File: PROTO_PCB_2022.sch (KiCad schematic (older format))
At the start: 19 parts, among them J1 HORN_EN1, J10 VESC_EN_SIGNAL, J11 BRAKELIGHTS_PWR_OUT, J12 HORN_PWR_OUT, J2 BRAKELIGHTS_EN1, J3 STARTER_MOTOR_EN, J4 12V_BATT1, J5 12V_EXTRA, J6 ECU_POWER_DIST, J7 ECU_KILL_1, J8 ECU_KILL_2, J9 ECU_KILL_3, K1 RT214012, Q1 BRAKELIGHTS_MOSFET1, Q2 HORN_MOSFET1

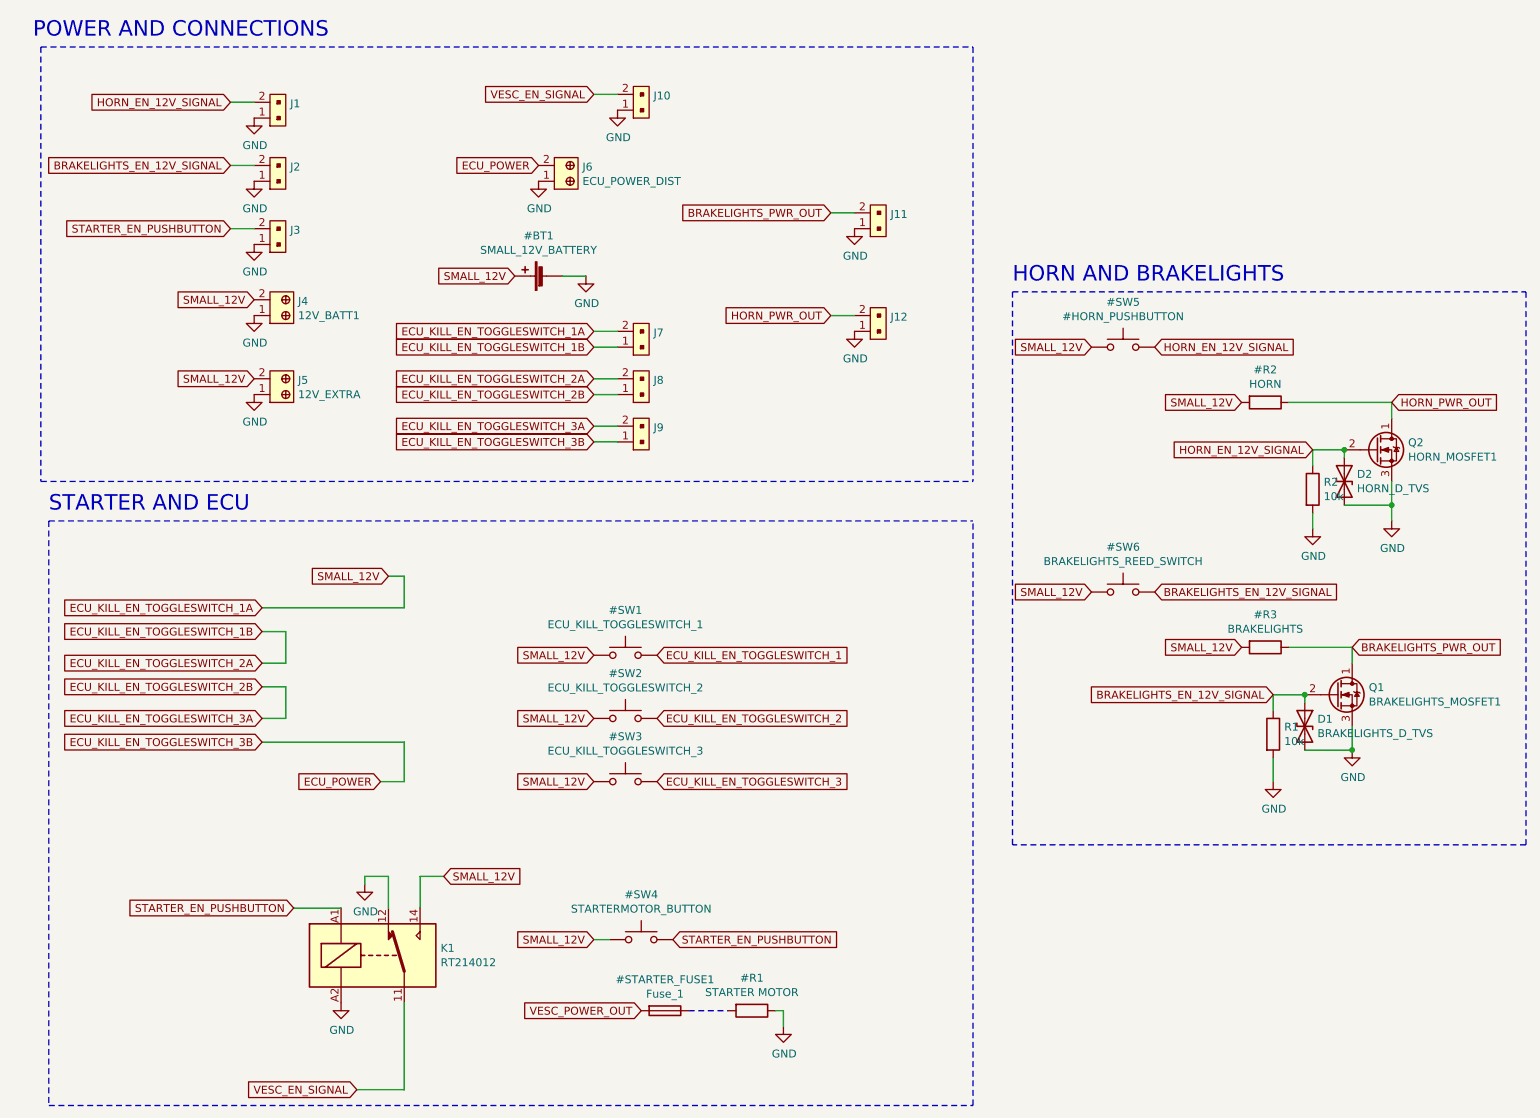
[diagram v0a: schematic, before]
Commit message: second version
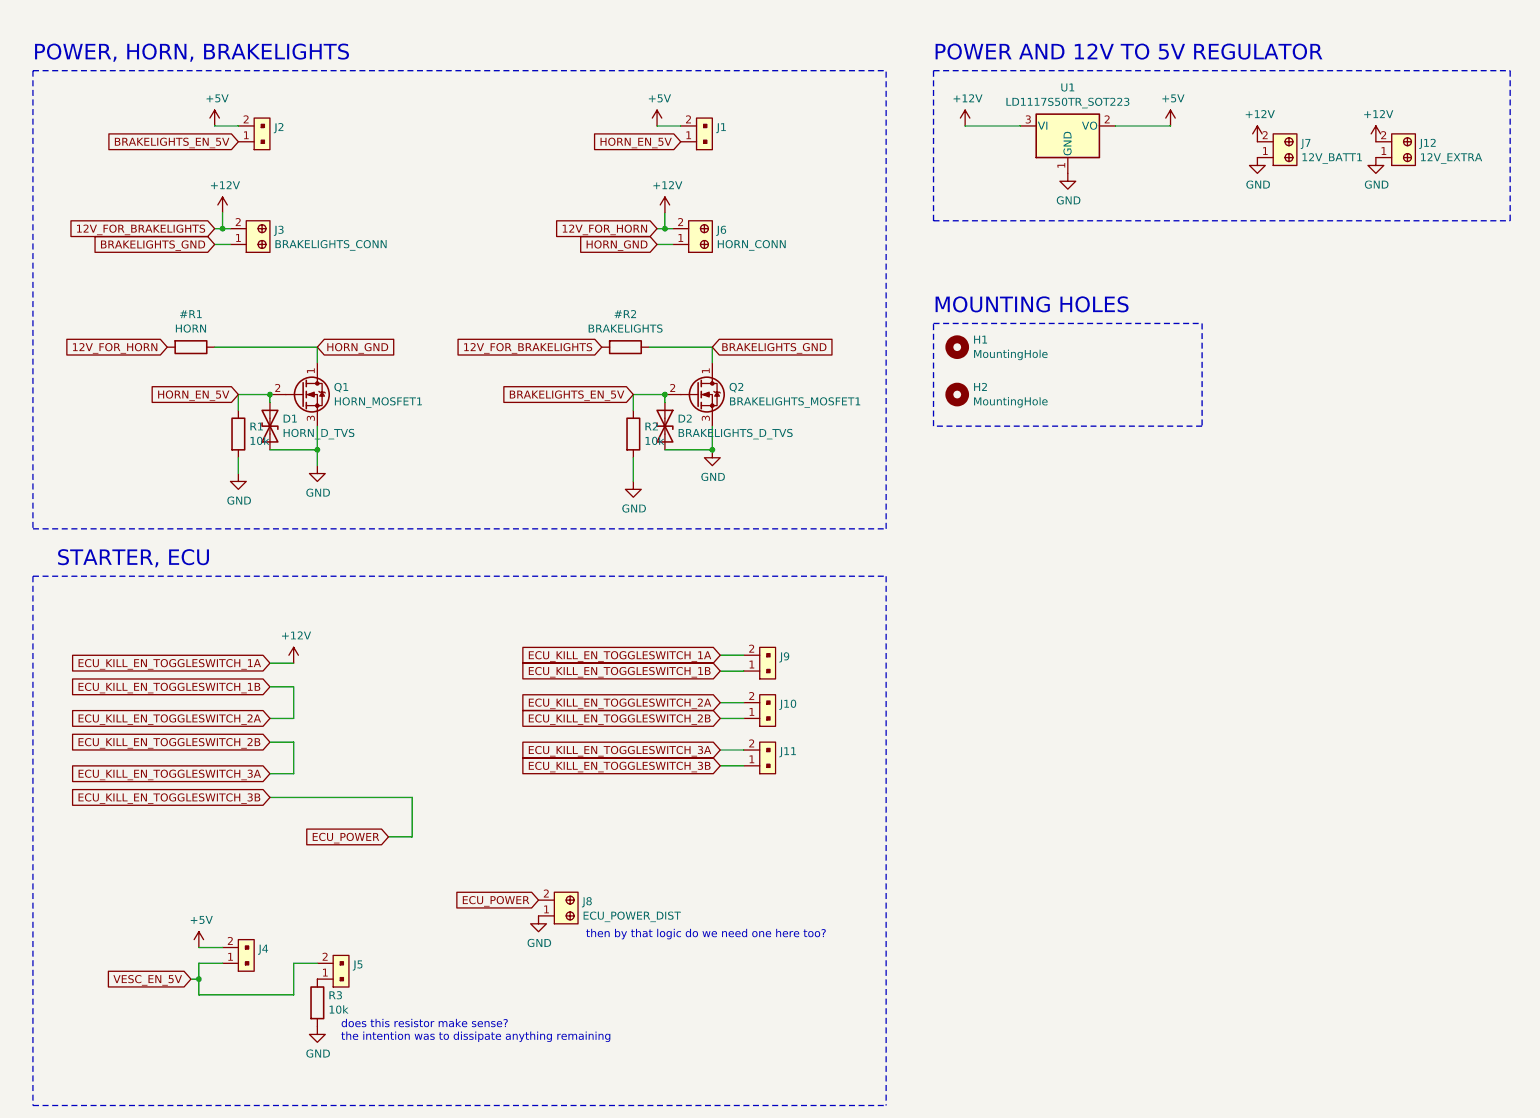
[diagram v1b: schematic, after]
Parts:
- removed J11: BRAKELIGHTS_PWR_OUT, Footprint Library:Molex_Proto_Microfit_Footprint, symbol PROTO_PCB_2022-rescue:B2B-PH-K-S_LF__SN_-dk_Rectangular-Connectors-Headers-Male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
- removed J12: HORN_PWR_OUT, Footprint Library:Molex_Proto_Microfit_Footprint, symbol PROTO_PCB_2022-rescue:B2B-PH-K-S_LF__SN_-dk_Rectangular-Connectors-Headers-Male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
- removed K1: RT214012, Relay_THT:Relay_SPDT_Schrack-RT1-FormC_RM5mm, symbol Relay:RT314A12
- added H1, H2: MountingHole, MountingHole:MountingHole_2.7mm_M2.5, symbol Mechanical:MountingHole
- added J3: BRAKELIGHTS_CONN, TerminalBlock_Phoenix:TerminalBlock_Phoenix_PT-1,5-2-5.0-H_1x02_P5.00mm_Horizontal, symbol PROTO_PCB_2022-rescue:1935161-dk_Terminal-Blocks-Wire-to-Board
- added J6: HORN_CONN, TerminalBlock_Phoenix:TerminalBlock_Phoenix_PT-1,5-2-5.0-H_1x02_P5.00mm_Horizontal, symbol PROTO_PCB_2022-rescue:1935161-dk_Terminal-Blocks-Wire-to-Board
- added R3: 10k, Resistor_SMD:R_0603_1608Metric, symbol Device:R
- added U1: LD1117S50TR_SOT223, Package_TO_SOT_SMD:SOT-223-3_TabPin2, symbol Regulator_Linear:LD1117S50TR_SOT223
- renumbered D2 to D1, D1 to D2, J8 to J10, J9 to J11, J5 to J12, J3 to J4, J10 to J5, J4 to J7, J6 to J8, J7 to J9, Q2 to Q1, Q1 to Q2, R2 to R1, R1 to R2
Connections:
- net GND: now also R3.2, U1.1 (GND); no longer J1.1, J2.1, J4.1, J5.1
- net BRAKELIGHTS_EN_12V_SIGNAL renamed BRAKELIGHTS_EN_5V
- net BRAKELIGHTS_EN_5V: now also J2.1; no longer J2.2
- net BRAKELIGHTS_PWR_OUT renamed BRAKELIGHTS_GND
- net BRAKELIGHTS_GND: now also J3.1
- net ECU_KILL_EN_TOGGLESWITCH_1A renamed +12V
- net +12V: now also J3.2, J6.2, U1.3 (VI)
- net HORN_EN_12V_SIGNAL renamed HORN_EN_5V
- net HORN_EN_5V: now also J1.1; no longer J1.2
- net HORN_PWR_OUT renamed HORN_GND
- net HORN_GND: now also J6.1
- net STARTER_EN_PUSHBUTTON renamed +5V
- net +5V: now also J1.2, J2.2, U1.2 (VO)
- net VESC_EN_SIGNAL renamed VESC_EN_5V
- net VESC_EN_5V: now also J4.1
- new net: J5.1, R3.1
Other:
- note added: "MOUNTING HOLES"
- note added: "POWER AND 12V TO 5V REGULATOR"
- note added: "POWER, HORN, BRAKELIGHTS"
- note added: "STARTER, ECU\n"
- note added: "does this resistor make sense?\nthe intention was to dissipate anything remaining"
- note added: "then by that logic do we need one here too?"
- note removed: "HORN AND BRAKELIGHTS"
- note removed: "POWER AND CONNECTIONS\n"
- note removed: "STARTER AND ECU\n"
- moved on the sheet: D1, D2, J1, J10, J11, J12, J2, J4, J5, J7, J8, J9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
